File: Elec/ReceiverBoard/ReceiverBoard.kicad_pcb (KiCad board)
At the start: 2 copper layers, 40 x 100 mm, 2 parts, among them J1 Conn_01x03, J2 Conn_01x03

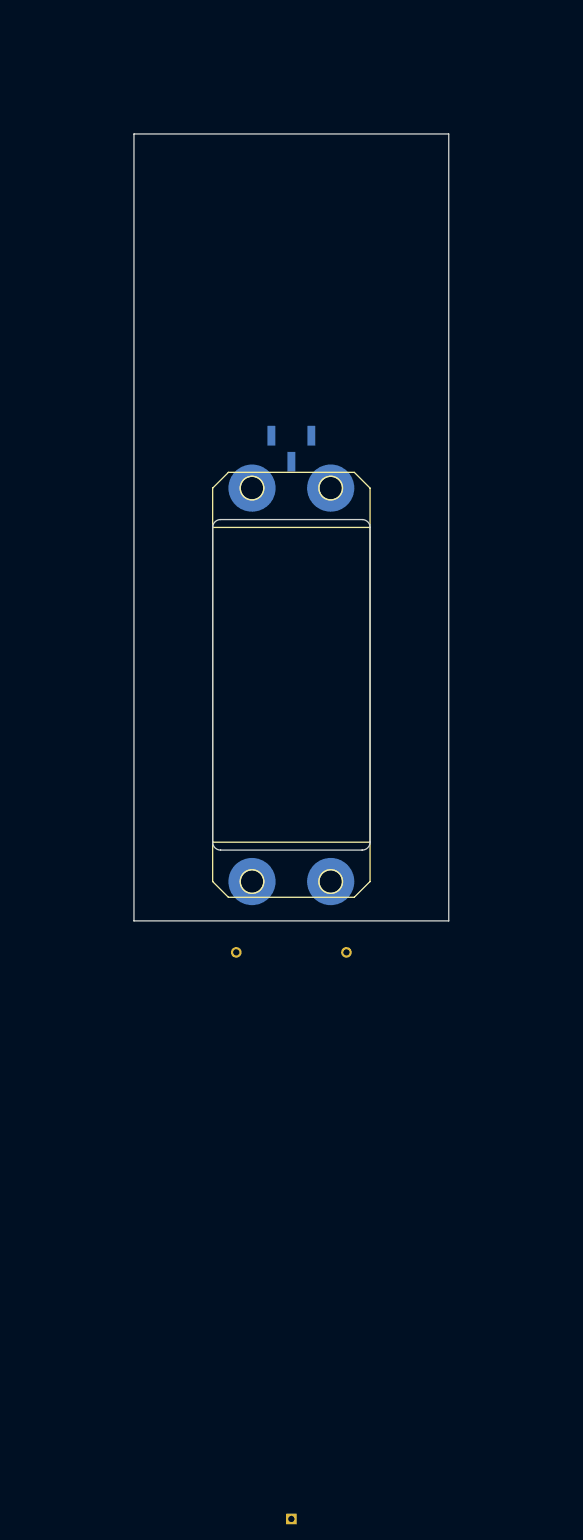
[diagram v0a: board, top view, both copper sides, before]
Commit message: SUKU ReceiverBoard created
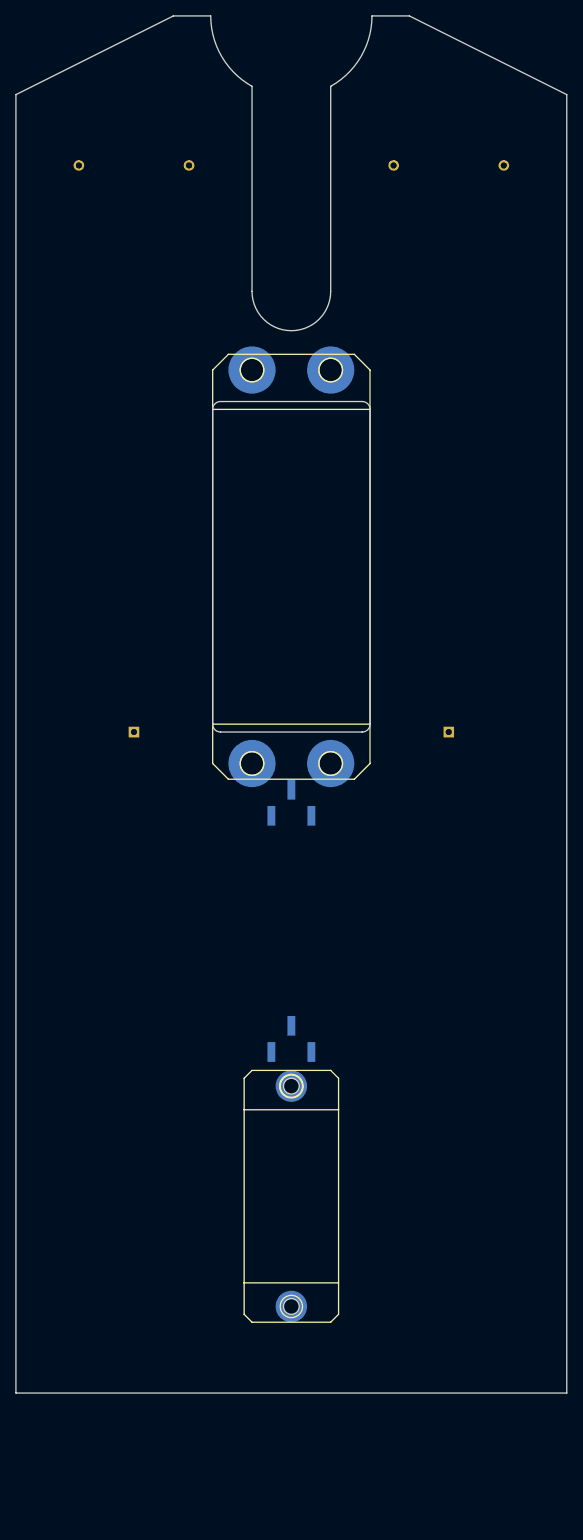
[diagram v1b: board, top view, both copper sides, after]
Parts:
- added J3: Conn_01x03, suku_basics:BATTERY_2X_18650, B.Cu at (80.0, 90.0)
- added J4: Conn_01x03, suku_basics:SERVO_MICRO, F.Cu at (100.0, 185.0)
- moved J2 102.0 mm to (120.0, 90.0)
- moved J1 15.0 mm to (100.0, 105.0), turned to 180 degrees
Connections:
- J1 pad 1: (no net) -> /ORANGE
- J1 pad 2: (no net) -> /RED
- J1 pad 3: (no net) -> /BLACK
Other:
- board size 40 x 100 mm -> 70 x 175 mm
